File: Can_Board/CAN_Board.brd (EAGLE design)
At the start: 57 x 41 mm, 18 parts, among them J1 22-05-7028-02, J2 22-05-7028-02, U11 MCP2561-E/SN, X1 MSTBA2, X11 5504F1-09S-02A-03

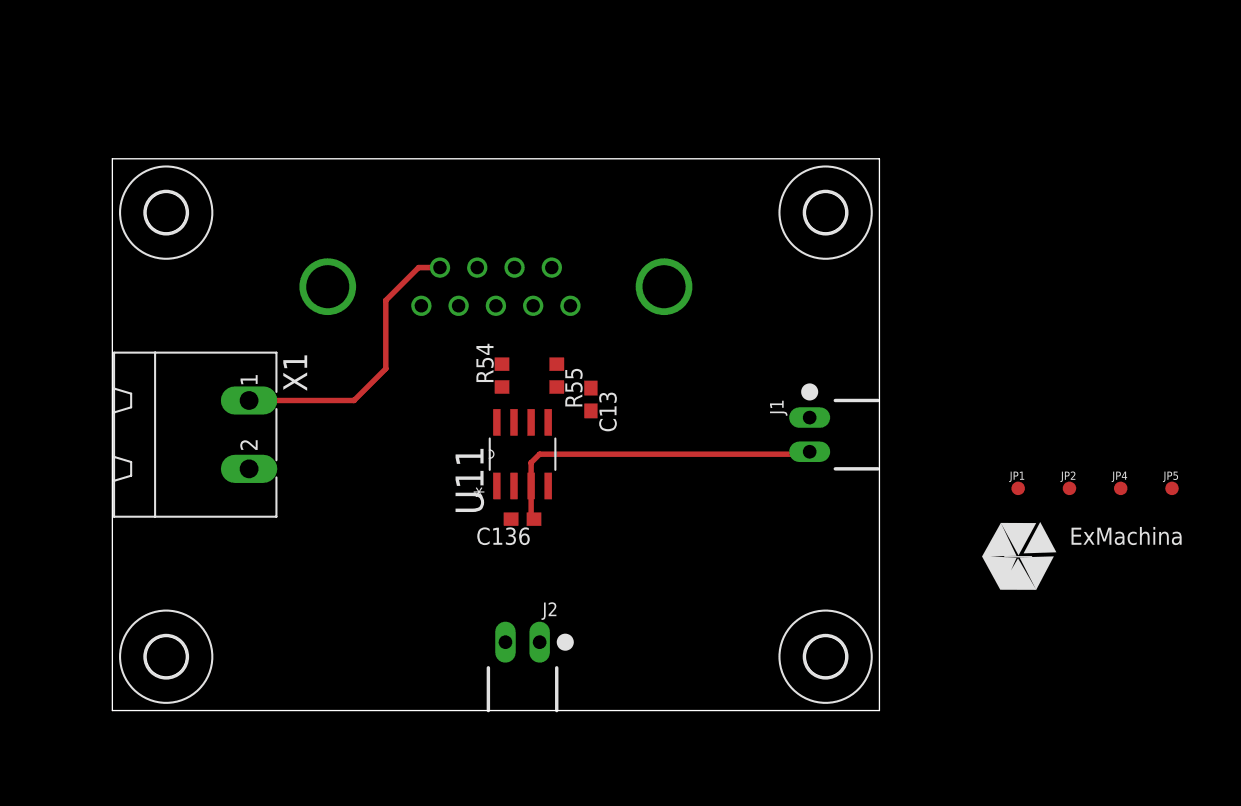
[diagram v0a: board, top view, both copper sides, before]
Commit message: Route the board
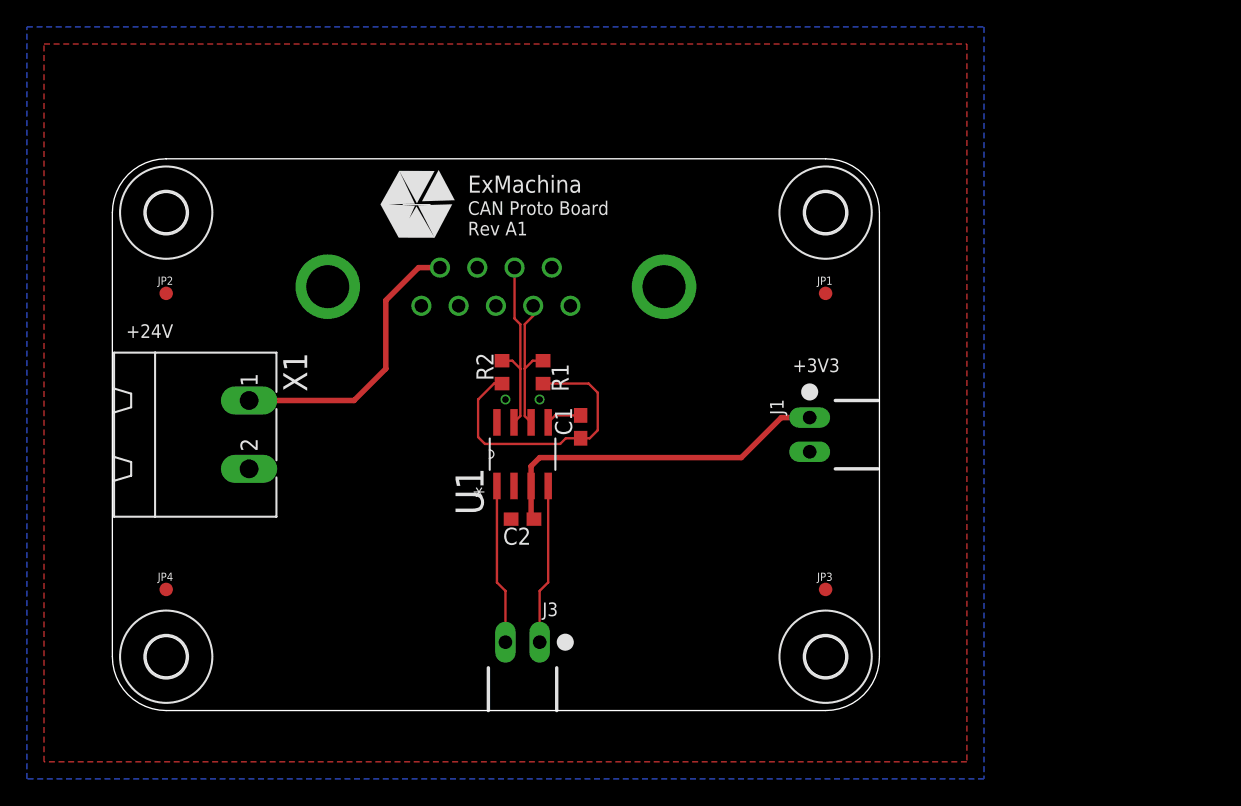
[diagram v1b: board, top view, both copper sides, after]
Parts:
- removed C13: 4700pF, rcl:C0603
- removed JP5: FIDUCIAL1X2, SparkFun:FIDUCIAL-1X2
- removed R54, R55: 60.4, rcl:R0603
- removed U$2: EXMACHINA-LOGO-NAME, exmachina:EXM-LOGO-BASELINE
- removed X11: 5504F1-09S-02A-03, con-multicomp:5504F1-09S-02A
- added C1: 4700pF, rcl:C0603
- added J3: 22-05-7028-02, con-molex:7395-02
- added JP3: FIDUCIAL1X2, SparkFun:FIDUCIAL-1X2
- added R1, R2: 60.4, rcl:R0603
- added T1: EXMACHINA-LOGO-NAME, exmachina:EXM-LOGO-BASELINE
- J2: value 22-05-7028-02 -> 5504F1-09S-02A-03; device con-molex:7395-02 -> con-multicomp:5504F1-09S-02A
- moved JP4 71.3 mm to (4.00, 9.00)
- moved JP2 68.7 mm to (4.00, 31.0)
- moved J2 26.5 mm to (28.5, 31.5), flipped to the bottom
- moved JP1 20.4 mm to (53.0, 31.0)
- renumbered C136 to C2, U11 to U1
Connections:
- net +24V: now also J2.9; no longer X11.9
- net +3V3: now also J1.1; no longer J1.2
- net CAN_N: now also J2.2, R1.1; no longer R55.1, X11.2
- net CAN_P: now also J2.7, R2.2; no longer R54.2, X11.7
- net CAN_RX: now also J3.1; no longer J2.1
- net CAN_SHLD: now also J2.5; no longer X11.5
- net CAN_SPLIT: now also C1.2; no longer C13.2
- net CAN_TX: now also J3.2; no longer J2.2
- net GND: now also J1.2, J2.3, J2.6; no longer J1.1, X11.3, X11.6
- net N$3: now also C1.1, R1.2, R2.1; no longer C13.1, R54.1, R55.2
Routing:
- net N$3: track 0.00 -> 21.7 mm
- net CAN_P: track 0.00 -> 13.5 mm
- net CAN_TX: track 0.00 -> 11.9 mm
- net CAN_RX: track 0.00 -> 11.9 mm
- net CAN_N: track 0.00 -> 10.7 mm
- net CAN_SPLIT: track 0.00 -> 2.63 mm
- net +3V3: track 25.4 -> 26.3 mm
- added copper zone on layer 1, net GND
- added copper zone on layer 16, net GND
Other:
- outline, holes or cut-outs redrawn
- board text added: "+24V"
- board text added: "+3V3"
- board text added: "CAN Proto Board Rev A1"
- board text added: "RX"
- board text added: "TX"
